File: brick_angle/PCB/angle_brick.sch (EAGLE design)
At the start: 2 parts, among them J1 3PIN, U1 ANGLE

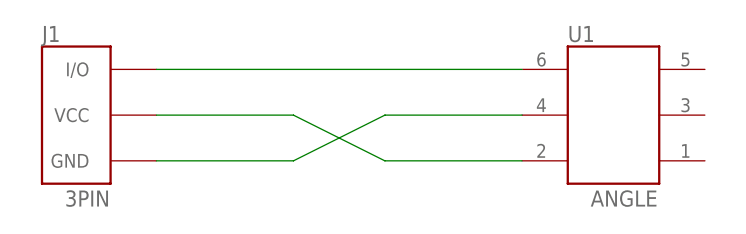
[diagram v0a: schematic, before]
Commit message: refine PCB board fix library
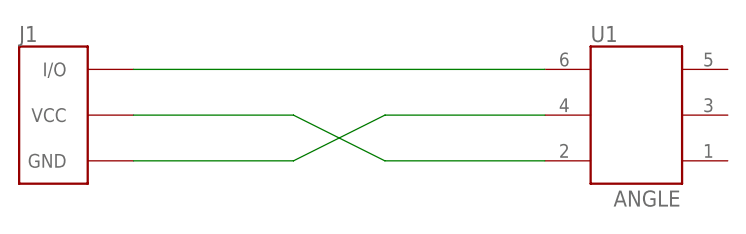
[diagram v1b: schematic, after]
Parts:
- J1: device fabo:BRICK_3PIN -> gclue:BRICK_3PIN
- U1: device fabo:BRICK_ANGLE -> gclue:ROTARYENCORDER_BRICK
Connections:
- net N$2 renamed VCC
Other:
- moved on the sheet: J1, U1
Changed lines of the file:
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@@
 <setting verticaltext="up"/>
 </settings>
-<grid distance="0.1" unitdist="inch" unit="inch" style="lines" multiple="1" display="yes" altdistance="0.01" altunitdist="inch" altunit="inch"/>
+<grid distance="0.1" unitdist="inch" unit="inch" style="lines" multiple="1" display="no" altdistance="0.01" altunitdist="inch" altunit="inch"/>
 <layers>
 <layer number="1" name="Top" color="4" fill="1" visible="no" active="no"/>
@@
 </classes>
 <parts>
-<part name="U$2" library="fabo" deviceset="A4L-LOC" device=""/>
-<part name="J1" library="fabo" deviceset="BRICK_3PIN" device="" value="3PIN"/>
-<part name="U1" library="fabo" deviceset="BRICK_ANGLE" device="" value="ANGLE"/>
+<part name="U$1" library="gclue" deviceset="A4L-LOC" device=""/>
+<part name="J1" library="gclue" deviceset="BRICK_3PIN" device="" value="3PIN"/>
+<part name="U1" library="gclue" deviceset="ROTARYENCORDER_BRICK" device="" value="ANGLE"/>
 </parts>
 <sheets>
@@
 </plain>
 <instances>
-<instance part="U$2" gate="G$1" x="0" y="0"/>
-<instance part="J1" gate="G$1" x="93.98" y="88.9" smashed="yes">
-<attribute name="NAME" x="88.9" y="97.028" size="1.778" layer="95"/>
-<attribute name="VALUE" x="91.44" y="78.74" size="1.778" layer="96"/>
+<instance part="U$1" gate="G$1" x="0" y="0"/>
+<instance part="J1" gate="G$1" x="91.44" y="88.9" smashed="yes">
+<attribute name="NAME" x="86.36" y="97.028" size="1.778" layer="95"/>
 </instance>
-<instance part="U1" gate="G$1" x="152.4" y="88.9" smashed="yes" rot="R180">
-<attribute name="NAME" x="147.32" y="97.028" size="1.778" layer="95"/>
-<attribute name="VALUE" x="149.86" y="78.74" size="1.778" layer="96"/>
+<instance part="U1" gate="G$1" x="154.94" y="88.9" smashed="yes" rot="R180">
+<attribute name="NAME" x="149.86" y="97.028" size="1.778" layer="95"/>
+<attribute name="VALUE" x="152.4" y="78.74" size="1.778" layer="96"/>
 </instance>
 </instances>
@@
 </busses>
 <nets>
-<net name="N$2" class="0">
+<net name="N$1" class="0">
 <segment>
-<wire x1="142.24" y1="83.82" x2="127" y2="83.82" width="0.1524" layer="91"/>
-<wire x1="127" y1="83.82" x2="116.84" y2="88.9" width="0.1524" layer="91"/>
-<wire x1="116.84" y1="88.9" x2="101.6" y2="88.9" width="0.1524" layer="91"/>
-<pinref part="J1" gate="G$1" pin="VCC"/>
-<pinref part="U1" gate="G$1" pin="2"/>
+<pinref part="J1" gate="G$1" pin="I/O"/>
+<pinref part="U1" gate="G$1" pin="6"/>
+<wire x1="99.06" y1="93.98" x2="144.78" y2="93.98" width="0.1524" layer="91"/>
 </segment>
 </net>
-<net name="N$1" class="0">
+<net name="VCC" class="0">
 <segment>
-<wire x1="101.6" y1="93.98" x2="142.24" y2="93.98" width="0.1524" layer="91"/>
-<pinref part="J1" gate="G$1" pin="I/O"/>
-<pinref part="U1" gate="G$1" pin="6"/>
+<pinref part="J1" gate="G$1" pin="VCC"/>
+<wire x1="99.06" y1="88.9" x2="116.84" y2="88.9" width="0.1524" layer="91"/>
+<wire x1="116.84" y1="88.9" x2="127" y2="83.82" width="0.1524" layer="91"/>
+<pinref part="U1" gate="G$1" pin="2"/>
+<wire x1="127" y1="83.82" x2="144.78" y2="83.82" width="0.1524" layer="91"/>
 </segment>
 </net>
 <net name="GND" class="0">
 <segment>
-<wire x1="142.24" y1="88.9" x2="127" y2="88.9" width="0.1524" layer="91"/>
-<wire x1="127" y1="88.9" x2="116.84" y2="83.82" width="0.1524" layer="91"/>
-<wire x1="116.84" y1="83.82" x2="101.6" y2="83.82" width="0.1524" layer="91"/>
 <pinref part="J1" gate="G$1" pin="GND"/>
+<wire x1="99.06" y1="83.82" x2="116.84" y2="83.82" width="0.1524" layer="91"/>
+<wire x1="116.84" y1="83.82" x2="127" y2="88.9" width="0.1524" layer="91"/>
 <pinref part="U1" gate="G$1" pin="4"/>
+<wire x1="127" y1="88.9" x2="144.78" y2="88.9" width="0.1524" layer="91"/>
 </segment>
 </net>
